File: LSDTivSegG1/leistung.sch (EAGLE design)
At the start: 86 parts, among them IC10 LM 2576 T15, IC11 LM 2576 T5.0, IC2 IR2184D, IC3 IR2184D, IC4 4081N, IC5 4069N, IC7 IR2184D, IC8 IR2184D, IC9 TINY13-20PU, Q1 IRFB3077, Q10 IRFB3077, Q11 IRFB3077, Q12 IRFB3077, Q2 IRFB3077, Q3 IRFB3077, Q4 IRFB3077, Q9 IRFB3077, X1 057-010-1, X2 MKDSN1,5/2-5,08

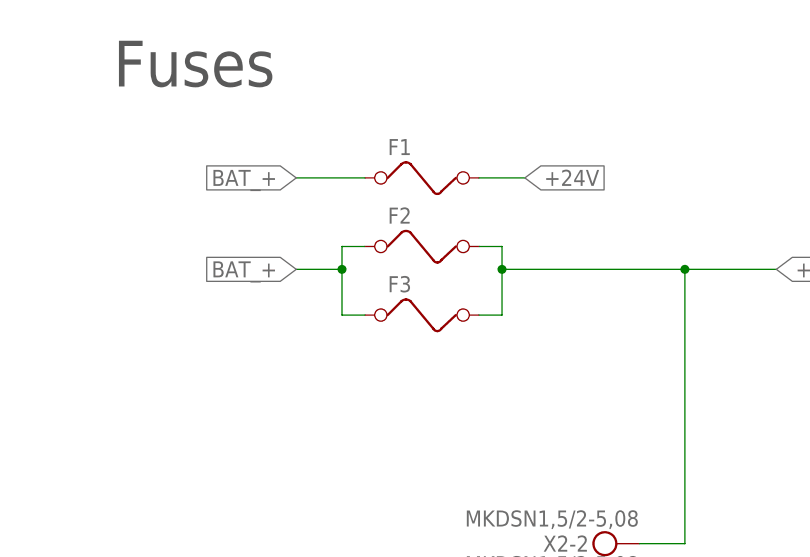
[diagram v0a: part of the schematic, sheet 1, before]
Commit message: added Text
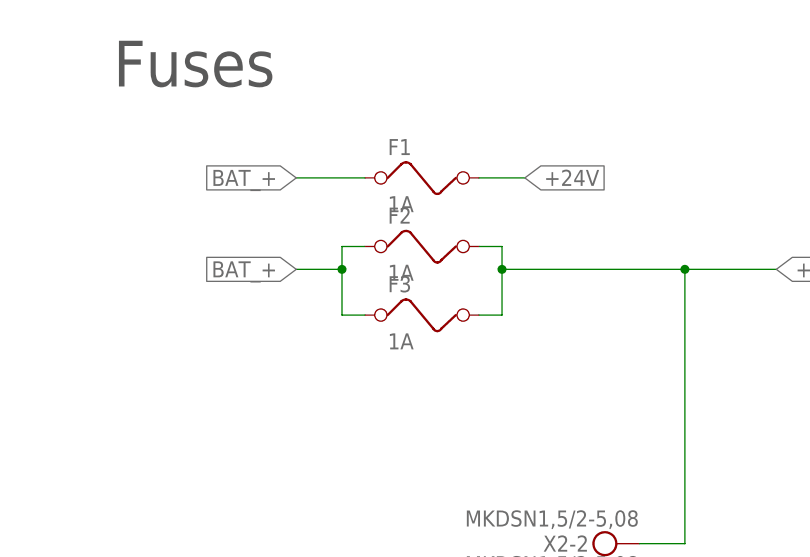
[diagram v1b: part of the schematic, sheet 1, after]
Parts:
- F1, F2, F3: value (none) -> 1A
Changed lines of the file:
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@@
 <grid distance="0.1" unitdist="inch" unit="inch" style="lines" multiple="1" display="no" altdistance="0.01" altunitdist="inch" altunit="inch"/>
 <layers>
-<layer number="1" name="Top" color="4" fill="1" visible="yes" active="no"/>
-<layer number="2" name="Route2" color="16" fill="1" visible="yes" active="no"/>
-<layer number="3" name="Route3" color="17" fill="1" visible="yes" active="no"/>
-<layer number="4" name="Route4" color="18" fill="1" visible="yes" active="no"/>
-<layer number="5" name="Route5" color="19" fill="1" visible="yes" active="no"/>
-<layer number="6" name="Route6" color="25" fill="1" visible="yes" active="no"/>
-<layer number="7" name="Route7" color="26" fill="1" visible="yes" active="no"/>
-<layer number="8" name="Route8" color="27" fill="1" visible="yes" active="no"/>
-<layer number="9" name="Route9" color="28" fill="1" visible="yes" active="no"/>
-<layer number="10" name="Route10" color="29" fill="1" visible="yes" active="no"/>
-<layer number="11" name="Route11" color="30" fill="1" visible="yes" active="no"/>
-<layer number="12" name="Route12" color="20" fill="1" visible="yes" active="no"/>
-<layer number="13" name="Route13" color="21" fill="1" visible="yes" active="no"/>
-<layer number="14" name="Route14" color="22" fill="1" visible="yes" active="no"/>
-<layer number="15" name="Route15" color="23" fill="1" visible="yes" active="no"/>
-<layer number="16" name="Bottom" color="1" fill="1" visible="yes" active="no"/>
-<layer number="17" name="Pads" color="2" fill="1" visible="yes" active="no"/>
-<layer number="18" name="Vias" color="2" fill="1" visible="yes" active="no"/>
-<layer number="19" name="Unrouted" color="6" fill="1" visible="yes" active="no"/>
-<layer number="20" name="Dimension" color="24" fill="1" visible="yes" active="no"/>
-<layer number="21" name="tPlace" color="7" fill="1" visible="yes" active="no"/>
-<layer number="22" name="bPlace" color="7" fill="1" visible="yes" active="no"/>
-<layer number="23" name="tOrigins" color="15" fill="1" visible="yes" active="no"/>
-<layer number="24" name="bOrigins" color="15" fill="1" visible="yes" active="no"/>
-<layer number="25" name="tNames" color="7" fill="1" visible="yes" active="no"/>
-<layer number="26" name="bNames" color="7" fill="1" visible="yes" active="no"/>
-<layer number="27" name="tValues" color="7" fill="1" visible="yes" active="no"/>
-<layer number="28" name="bValues" color="7" fill="1" visible="yes" active="no"/>
+<layer number="1" name="Top" color="4" fill="1" visible="no" active="no"/>
+<layer number="2" name="Route2" color="16" fill="1" visible="no" active="no"/>
+<layer number="3" name="Route3" color="17" fill="1" visible="no" active="no"/>
+<layer number="4" name="Route4" color="18" fill="1" visible="no" active="no"/>
+<layer number="5" name="Route5" color="19" fill="1" visible="no" active="no"/>
+<layer number="6" name="Route6" color="25" fill="1" visible="no" active="no"/>
+<layer number="7" name="Route7" color="26" fill="1" visible="no" active="no"/>
+<layer number="8" name="Route8" color="27" fill="1" visible="no" active="no"/>
+<layer number="9" name="Route9" color="28" fill="1" visible="no" active="no"/>
+<layer number="10" name="Route10" color="29" fill="1" visible="no" active="no"/>
+<layer number="11" name="Route11" color="30" fill="1" visible="no" active="no"/>
+<layer number="12" name="Route12" color="20" fill="1" visible="no" active="no"/>
+<layer number="13" name="Route13" color="21" fill="1" visible="no" active="no"/>
+<layer number="14" name="Route14" color="22" fill="1" visible="no" active="no"/>
+<layer number="15" name="Route15" color="23" fill="1" visible="no" active="no"/>
+<layer number="16" name="Bottom" color="1" fill="1" visible="no" active="no"/>
+<layer number="17" name="Pads" color="2" fill="1" visible="no" active="no"/>
+<layer number="18" name="Vias" color="2" fill="1" visible="no" active="no"/>
+<layer number="19" name="Unrouted" color="6" fill="1" visible="no" active="no"/>
+<layer number="20" name="Dimension" color="24" fill="1" visible="no" active="no"/>
+<layer number="21" name="tPlace" color="7" fill="1" visible="no" active="no"/>
+<layer number="22" name="bPlace" color="7" fill="1" visible="no" active="no"/>
+<layer number="23" name="tOrigins" color="15" fill="1" visible="no" active="no"/>
+<layer number="24" name="bOrigins" color="15" fill="1" visible="no" active="no"/>
+<layer number="25" name="tNames" color="7" fill="1" visible="no" active="no"/>
+<layer number="26" name="bNames" color="7" fill="1" visible="no" active="no"/>
+<layer number="27" name="tValues" color="7" fill="1" visible="no" active="no"/>
+<layer number="28" name="bValues" color="7" fill="1" visible="no" active="no"/>
 <layer number="29" name="tStop" color="7" fill="3" visible="no" active="no"/>
 <layer number="30" name="bStop" color="7" fill="6" visible="no" active="no"/>
@@
 <layer number="35" name="tGlue" color="7" fill="4" visible="no" active="no"/>
 <layer number="36" name="bGlue" color="7" fill="5" visible="no" active="no"/>
-<layer number="37" name="tTest" color="7" fill="1" visible="yes" active="no"/>
-<layer number="38" name="bTest" color="7" fill="1" visible="yes" active="no"/>
+<layer number="37" name="tTest" color="7" fill="1" visible="no" active="no"/>
+<layer number="38" name="bTest" color="7" fill="1" visible="no" active="no"/>
 <layer number="39" name="tKeepout" color="4" fill="11" visible="no" active="no"/>
 <layer number="40" name="bKeepout" color="1" fill="11" visible="no" active="no"/>
@@
 <layer number="44" name="Drills" color="7" fill="1" visible="no" active="no"/>
 <layer number="45" name="Holes" color="7" fill="1" visible="no" active="no"/>
-<layer number="46" name="Milling" color="3" fill="1" visible="yes" active="no"/>
-<layer number="47" name="Measures" color="7" fill="1" visible="yes" active="no"/>
-<layer number="48" name="Document" color="7" fill="1" visible="yes" active="no"/>
-<layer number="49" name="Reference" color="7" fill="1" visible="yes" active="no"/>
-<layer number="50" name="dxf" color="7" fill="1" visible="yes" active="no"/>
-<layer number="51" name="tDocu" color="7" fill="1" visible="yes" active="no"/>
-<layer number="52" name="bDocu" color="7" fill="1" visible="yes" active="no"/>
-<layer number="53" name="tGND_GNDA" color="7" fill="9" visible="yes" active="no"/>
-<layer number="54" name="bGND_GNDA" color="1" fill="9" visible="yes" active="no"/>
-<layer number="56" name="wert" color="7" fill="1" visible="yes" active="no"/>
+<layer number="46" name="Milling" color="3" fill="1" visible="no" active="no"/>
+<layer number="47" name="Measures" color="7" fill="1" visible="no" active="no"/>
+<layer number="48" name="Document" color="7" fill="1" visible="no" active="no"/>
+<layer number="49" name="Reference" color="7" fill="1" visible="no" active="no"/>
+<layer number="50" name="dxf" color="7" fill="1" visible="no" active="no"/>
+<layer number="51" name="tDocu" color="7" fill="1" visible="no" active="no"/>
+<layer number="52" name="bDocu" color="7" fill="1" visible="no" active="no"/>
+<layer number="53" name="tGND_GNDA" color="7" fill="9" visible="no" active="no"/>
+<layer number="54" name="bGND_GNDA" color="1" fill="9" visible="no" active="no"/>
+<layer number="56" name="wert" color="7" fill="1" visible="no" active="no"/>
 <layer number="88" name="SimResults" color="9" fill="1" visible="yes" active="yes"/>
 <layer number="89" name="SimProbes" color="9" fill="1" visible="yes" active="yes"/>
@@
 <part name="IC4" library="40xx" library_urn="urn:adsk.eagle:library:80" deviceset="4081" device="N" package3d_urn="urn:adsk.eagle:package:820/2"/>
 <part name="IC5" library="40xx" library_urn="urn:adsk.eagle:library:80" deviceset="4069" device="N" package3d_urn="urn:adsk.eagle:package:820/2"/>
-<part name="F1" library="special" library_urn="urn:adsk.eagle:library:367" deviceset="FUSE" device="" package3d_urn="urn:adsk.eagle:package:26650/1"/>
-<part name="F2" library="special" library_urn="urn:adsk.eagle:library:367" deviceset="FUSE" device="" package3d_urn="urn:adsk.eagle:package:26650/1"/>
-<part name="F3" library="special" library_urn="urn:adsk.eagle:library:367" deviceset="FUSE" device="" package3d_urn="urn:adsk.eagle:package:26650/1"/>
+<part name="F1" library="special" library_urn="urn:adsk.eagle:library:367" deviceset="FUSE" device="" package3d_urn="urn:adsk.eagle:package:26650/1" value="1A"/>
+<part name="F2" library="special" library_urn="urn:adsk.eagle:library:367" deviceset="FUSE" device="" package3d_urn="urn:adsk.eagle:package:26650/1" value="1A"/>
+<part name="F3" library="special" library_urn="urn:adsk.eagle:library:367" deviceset="FUSE" device="" package3d_urn="urn:adsk.eagle:package:26650/1" value="1A"/>
 <part name="X2" library="con-phoenix-508" library_urn="urn:adsk.eagle:library:176" deviceset="MKDSN1,5/2-5,08" device="" package3d_urn="urn:adsk.eagle:package:9630/1"/>
 <part name="FRAME5" library="frames" library_urn="urn:adsk.eagle:library:229" deviceset="DINA4_L" device=""/>
